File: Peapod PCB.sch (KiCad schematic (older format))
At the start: 16 parts, among them J1 CONN_01X01, J2 CONN_01X02, J3 CONN_01X01, J4 CONN_01X01, J5 CONN_01X01, J6 CONN_01X01, J7 CONN_01X02, U1 ESP8266

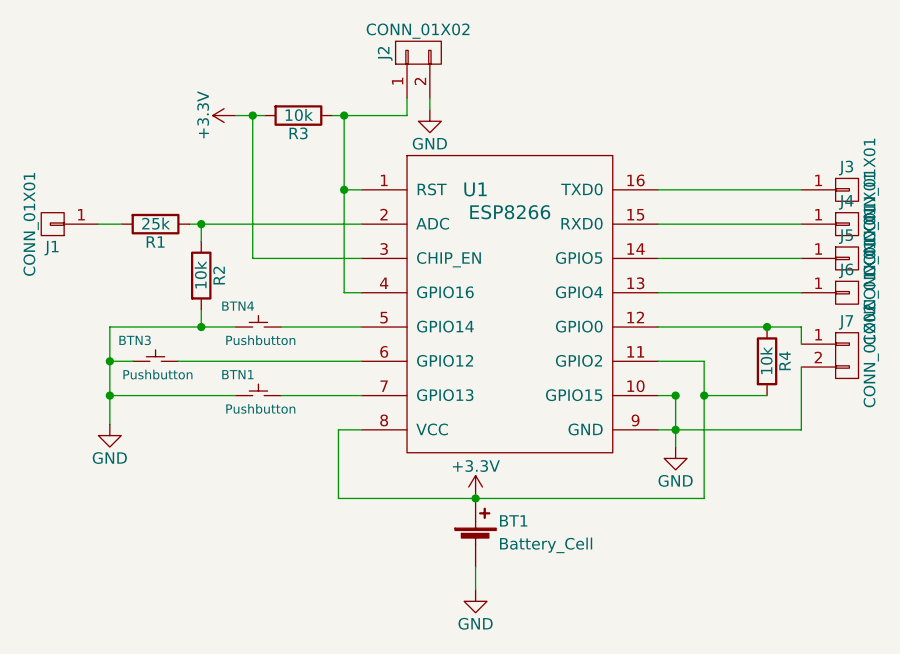
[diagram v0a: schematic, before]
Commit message: fixed changes
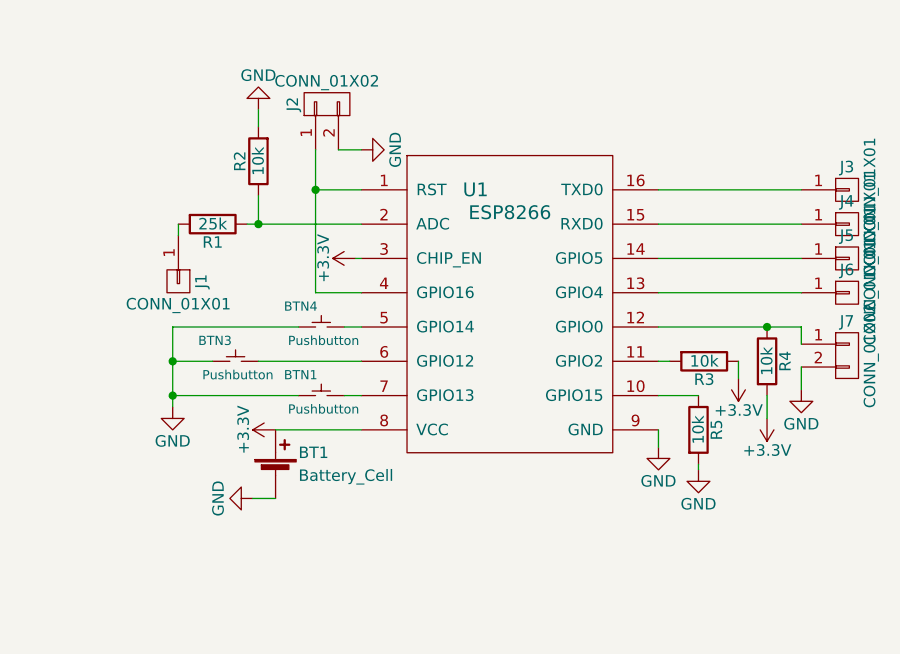
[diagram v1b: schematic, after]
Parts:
- added R5: 10k, symbol R
- R3: footprint Resistors_SMD:R_0805_HandSoldering -> (none)
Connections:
- net +3V3: now also R3.1; no longer R3.2, U1.11 (GPIO2)
- net GND: now also R5.2; no longer U1.10 (GPIO15)
- net at J2.1 (P1), U1.1 (RST), U1.4 (GPIO16): no longer R3.1
- new net: R5.1, U1.10 (GPIO15)
- new net: R3.2, U1.11 (GPIO2)
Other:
- moved on the sheet: BT1, BTN1, BTN3, BTN4, J1, J2, R1, R2
